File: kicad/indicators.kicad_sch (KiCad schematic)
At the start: 36 parts, among them J9 Free pin, U14 74LS244

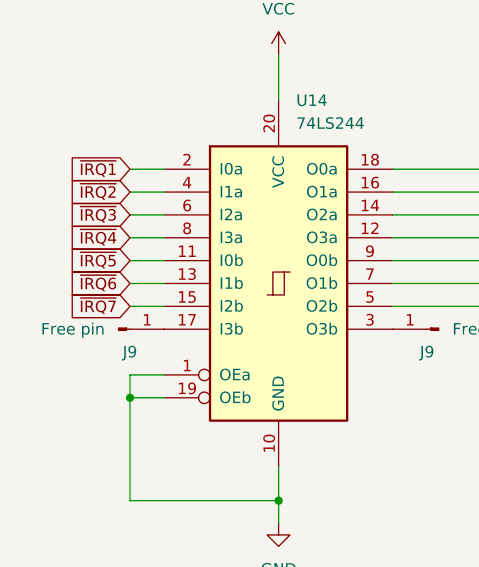
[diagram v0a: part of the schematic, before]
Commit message: saving kicad
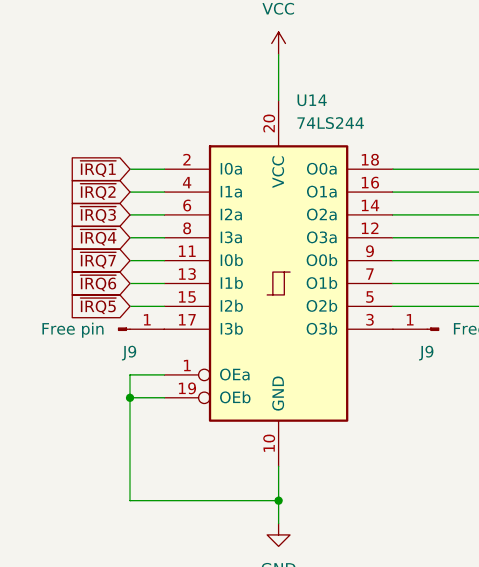
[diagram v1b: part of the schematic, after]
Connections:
- net ~{IRQ5}: now also U14.15 (I2b); no longer U14.11 (I0b)
- net ~{IRQ7}: now also U14.11 (I0b); no longer U14.15 (I2b)
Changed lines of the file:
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@@
     )
   )
-  (global_label "~{IRQ5}" (shape input) (at 85.09 45.72 180) (fields_autoplaced)
+  (global_label "~{IRQ5}" (shape input) (at 85.09 50.8 180) (fields_autoplaced)
     (effects (font (size 1.27 1.27)) (justify right))
-    (property "Intersheetrefs" "${INTERSHEET_REFS}" (at 77.7694 45.72 0)
+    (property "Intersheetrefs" "${INTERSHEET_REFS}" (at 77.7694 50.8 0)
       (effects (font (size 1.27 1.27)) (justify right) hide)
     )
@@
     )
   )
-  (global_label "~{IRQ7}" (shape input) (at 85.09 50.8 180) (fields_autoplaced)
+  (global_label "~{IRQ7}" (shape input) (at 85.09 45.72 180) (fields_autoplaced)
     (effects (font (size 1.27 1.27)) (justify right))
-    (property "Intersheetrefs" "${INTERSHEET_REFS}" (at 77.7694 50.8 0)
+    (property "Intersheetrefs" "${INTERSHEET_REFS}" (at 77.7694 45.72 0)
       (effects (font (size 1.27 1.27)) (justify right) hide)
     )
